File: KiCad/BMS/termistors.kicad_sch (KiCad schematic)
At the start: 19 parts, among them J6 430450800, J7 430450800, U21 74HC4051, U22 MCP3201, U23 HCPL-0630

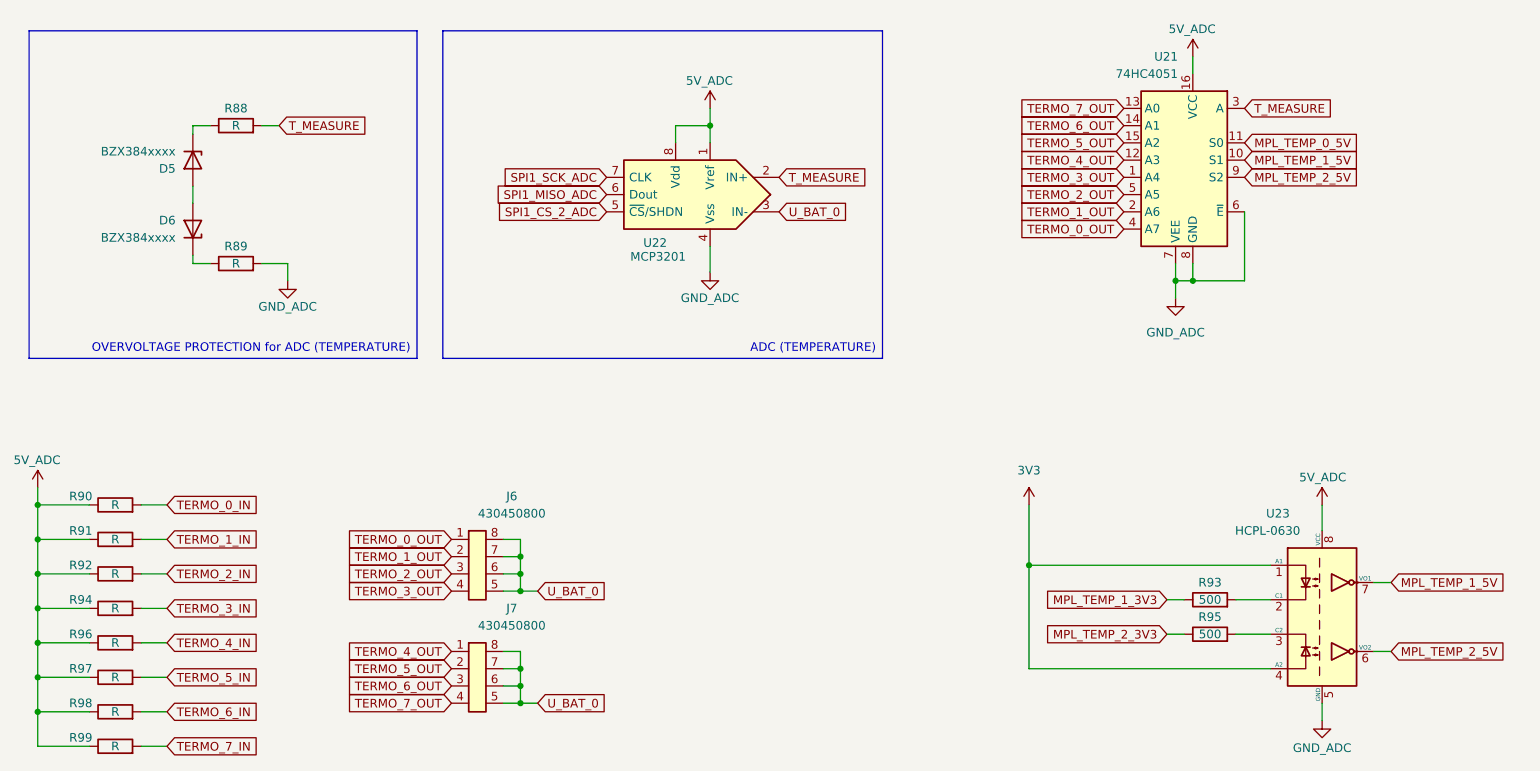
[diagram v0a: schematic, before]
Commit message: 27.03.2025
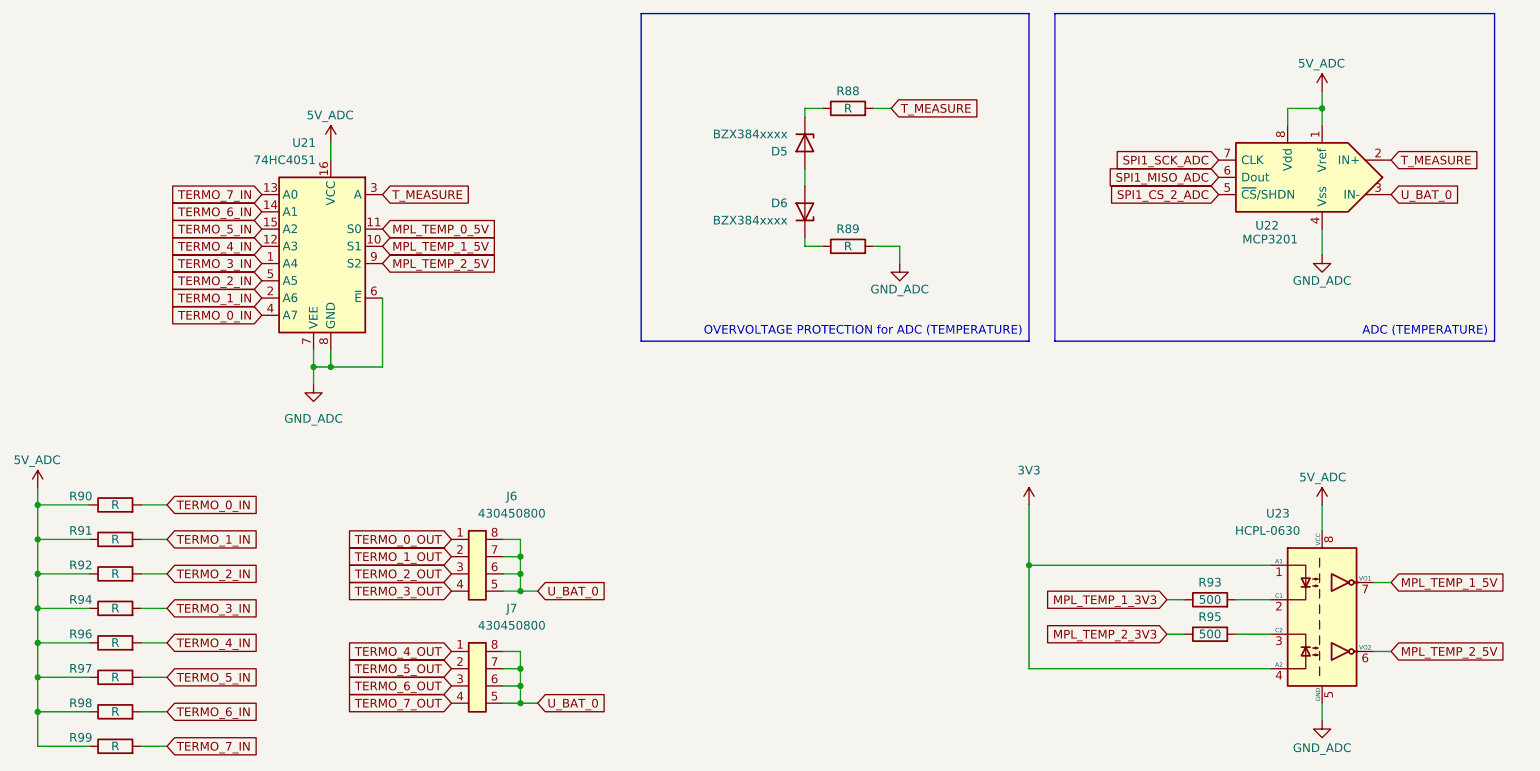
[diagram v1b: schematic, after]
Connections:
- net TERMO_0_IN: now also U21.4 (A7)
- net TERMO_0_OUT: no longer U21.4 (A7)
- net TERMO_1_IN: now also U21.2 (A6)
- net TERMO_1_OUT: no longer U21.2 (A6)
- net TERMO_2_IN: now also U21.5 (A5)
- net TERMO_2_OUT: no longer U21.5 (A5)
- net TERMO_3_IN: now also U21.1 (A4)
- net TERMO_3_OUT: no longer U21.1 (A4)
- net TERMO_4_IN: now also U21.12 (A3)
- net TERMO_4_OUT: no longer U21.12 (A3)
- net TERMO_5_IN: now also U21.15 (A2)
- net TERMO_5_OUT: no longer U21.15 (A2)
- net TERMO_6_IN: now also U21.14 (A1)
- net TERMO_6_OUT: no longer U21.14 (A1)
- net TERMO_7_IN: now also U21.13 (A0)
- net TERMO_7_OUT: no longer U21.13 (A0)
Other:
- moved on the sheet: D5, D6, R88, R89, U21, U22
